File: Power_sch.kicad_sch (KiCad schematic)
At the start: 53 parts, among them IC4 LM66200DRLR, J1 USB_C_Receptacle_USB2.0_16P, J8 USB_C_Receptacle_USB2.0_16P, Q3 BC849, Q4 BC849, U1 MIC5205-3.3YM5, U2 TPD2EUSB30ADRTR, U7 IR3883MTRPBF

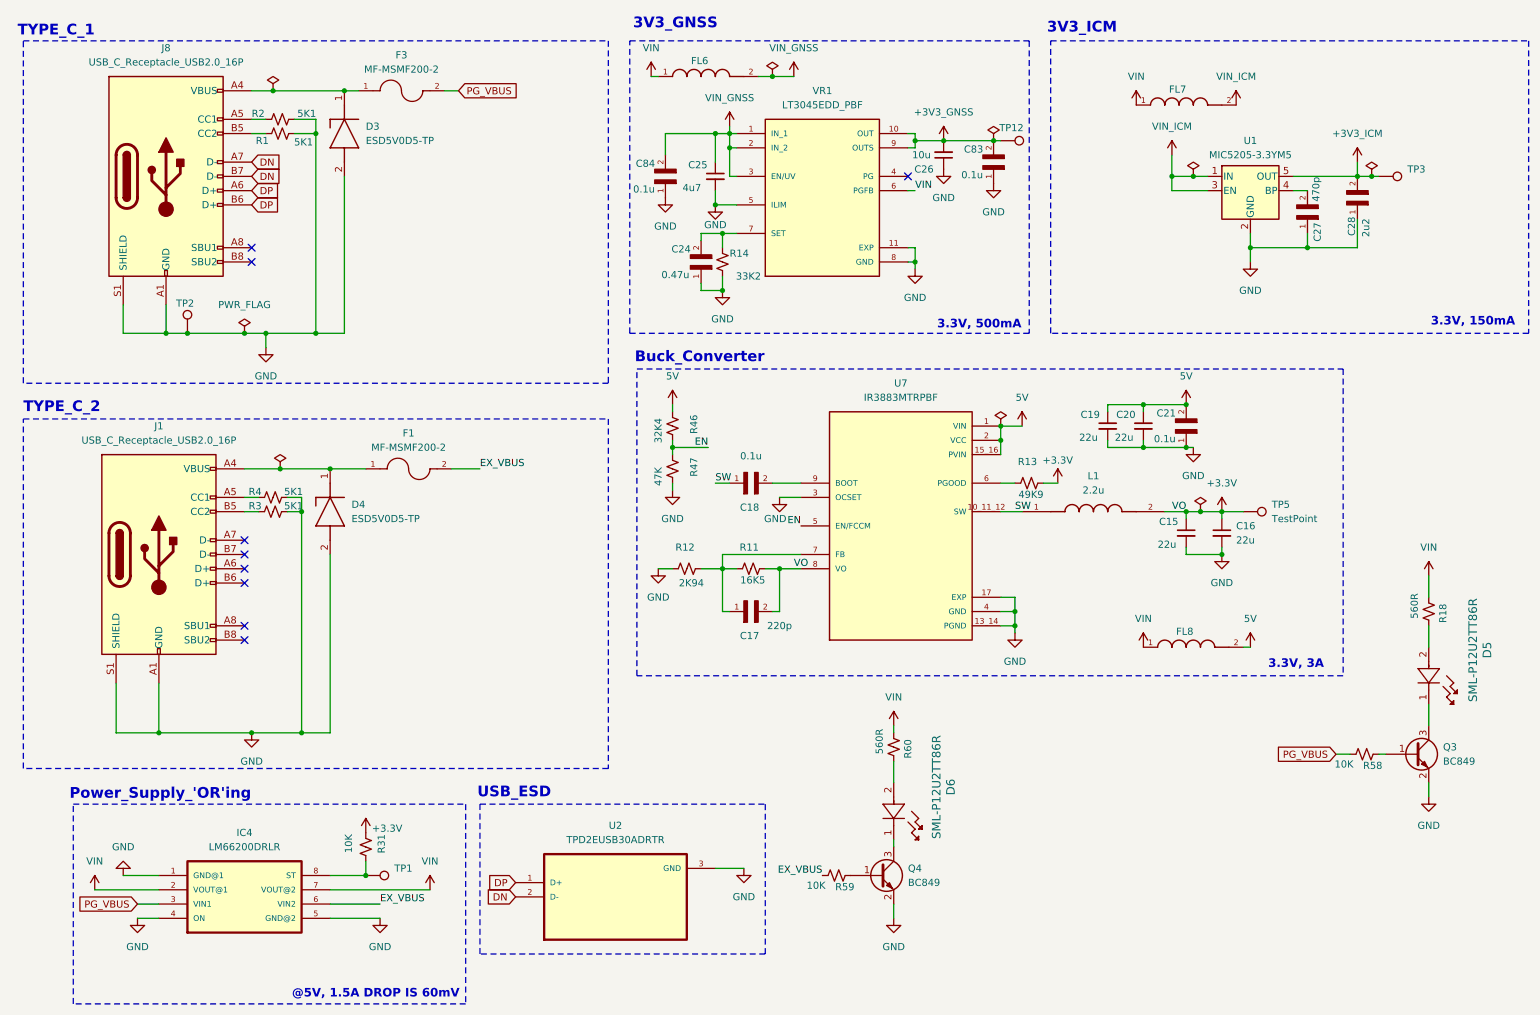
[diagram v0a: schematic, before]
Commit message: block
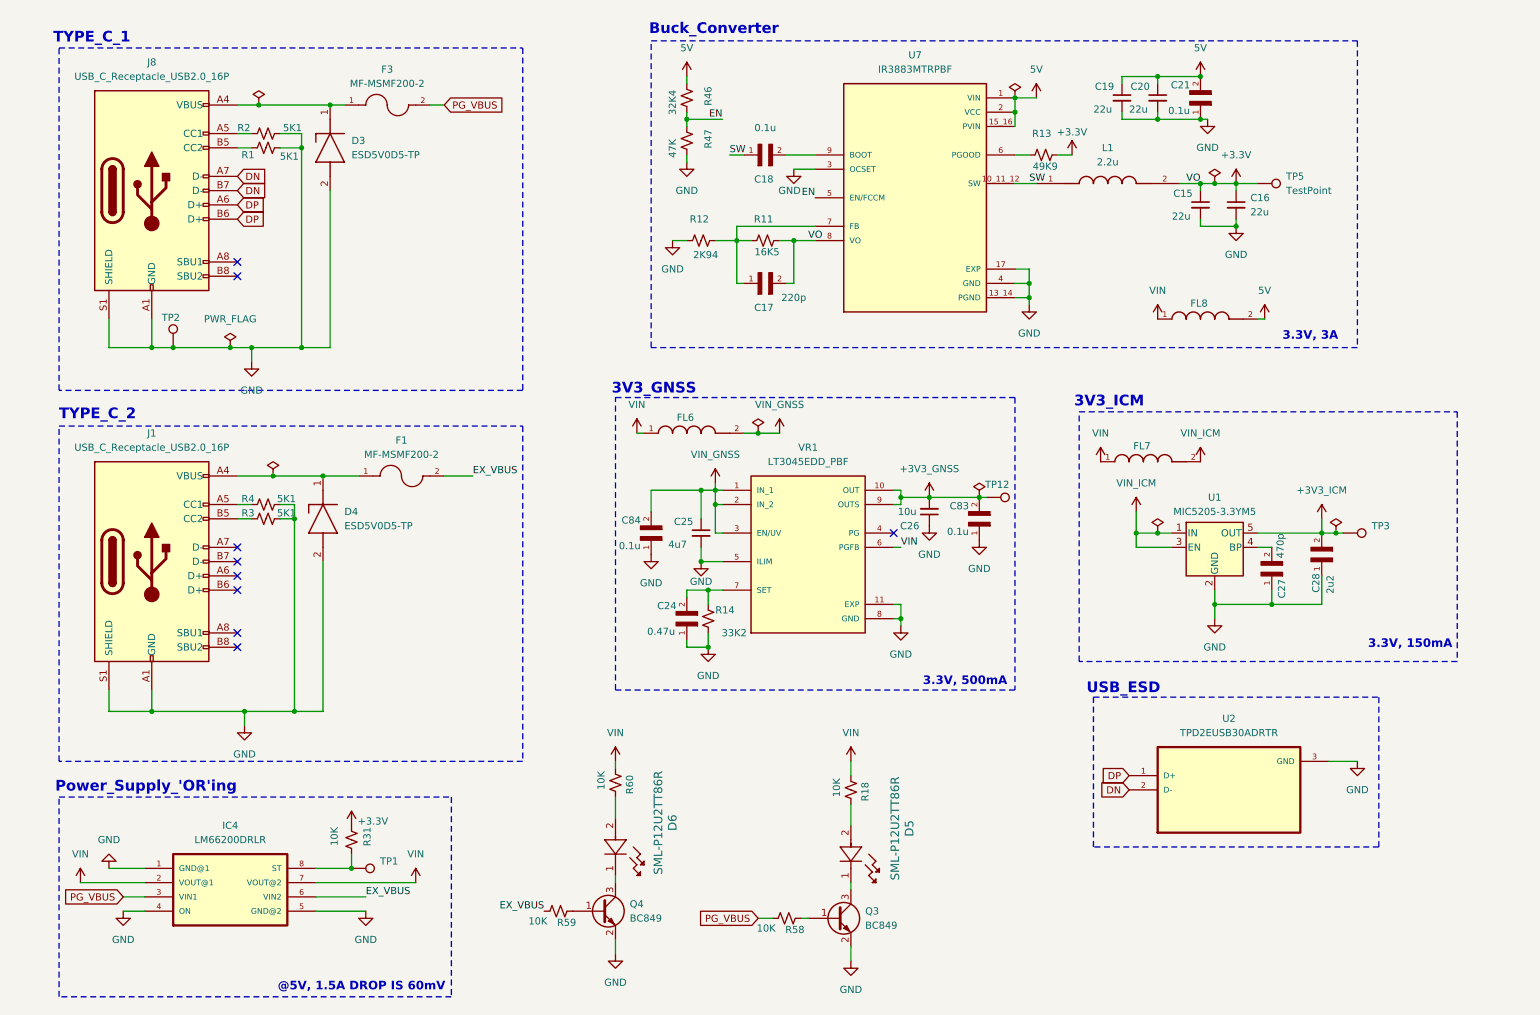
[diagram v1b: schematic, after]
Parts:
- R18, R60: value 560R -> 10K
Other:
- moved on the sheet: C15, C16, C17, C18, C19, C20, C21, C24, C25, C26, C27, C28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

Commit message: full
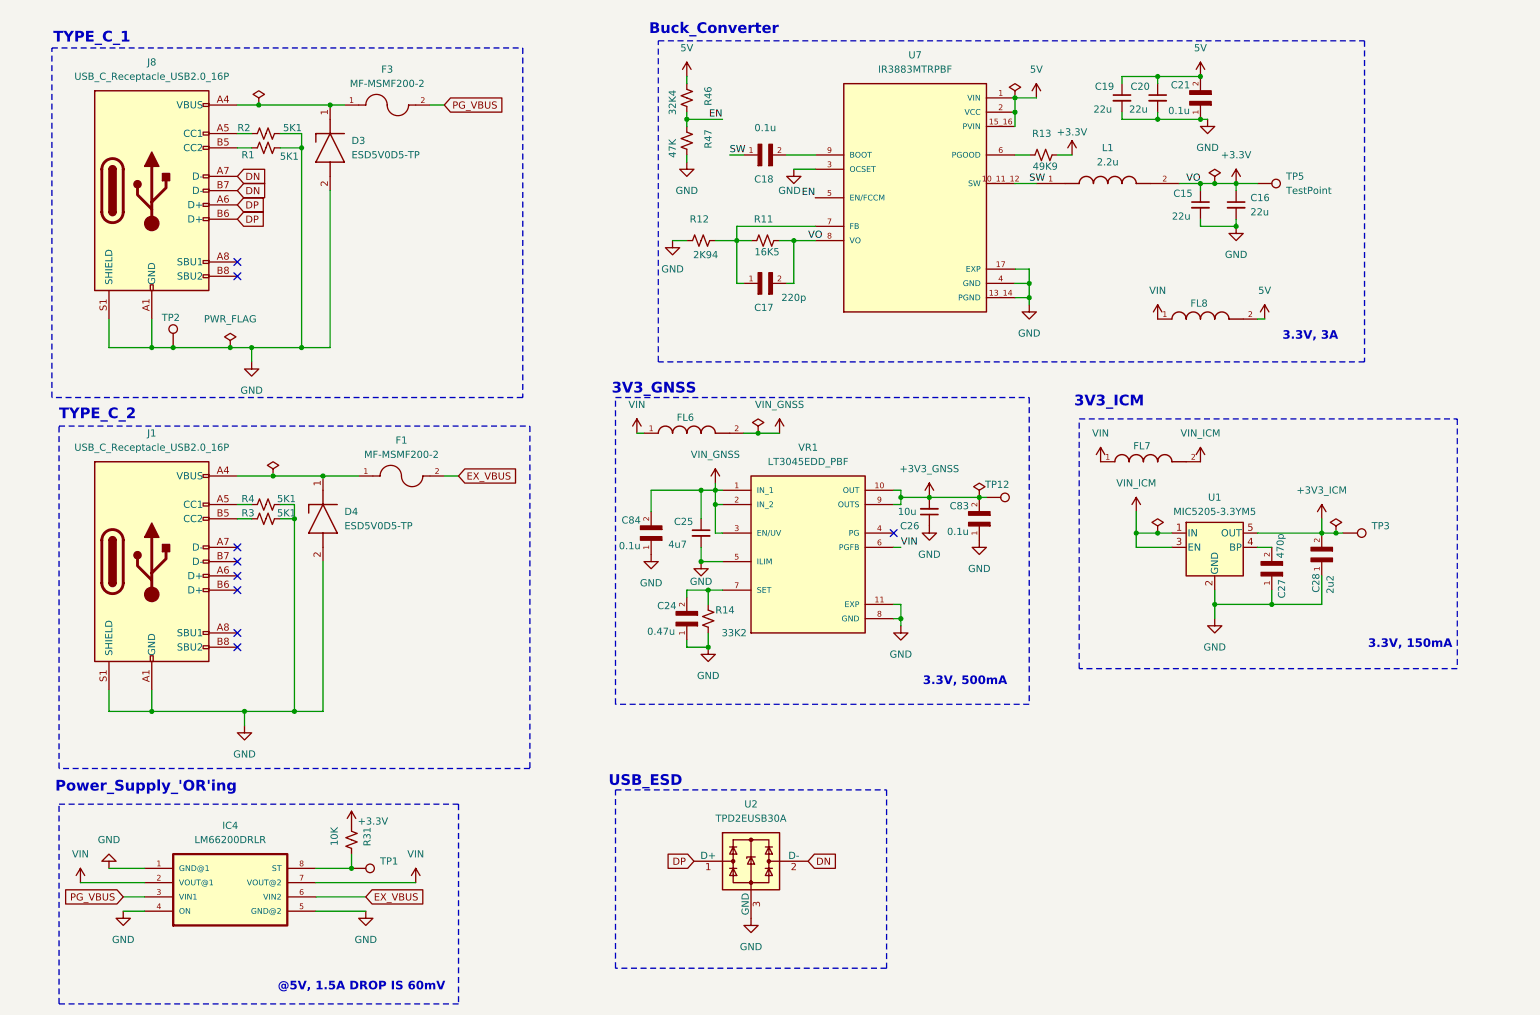
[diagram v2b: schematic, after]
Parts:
- removed D5, D6: SML-P12U2TT86R, LED_SMD:LED_0402_1005Metric, symbol 2026-08-14_04-34-19:SML-P12U2TT86R
- removed Q3, Q4: BC849, Package_TO_SOT_SMD:SOT-23, symbol Transistor_BJT:BC849
- removed R18, R58, R59, R60: 10K, Resistor_SMD:R_0402_1005Metric, symbol Device:R_Small_US
- removed U2: TPD2EUSB30ADRTR, GNSS:SOTFL35P100X50-3N, symbol TPD2EUSB30ADRTR:TPD2EUSB30ADRTR
- added U2: TPD2EUSB30A, Package_TO_SOT_SMD:Texas_DRT-3, symbol Power_Protection:TPD2EUSB30A
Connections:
- net DN: now also U2.2 (D-)
- net DP: now also U2.1 (D+)
- net GND: now also U2.3 (GND)
